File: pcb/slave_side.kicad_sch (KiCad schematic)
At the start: 2 parts, among them J6 AudioJack4

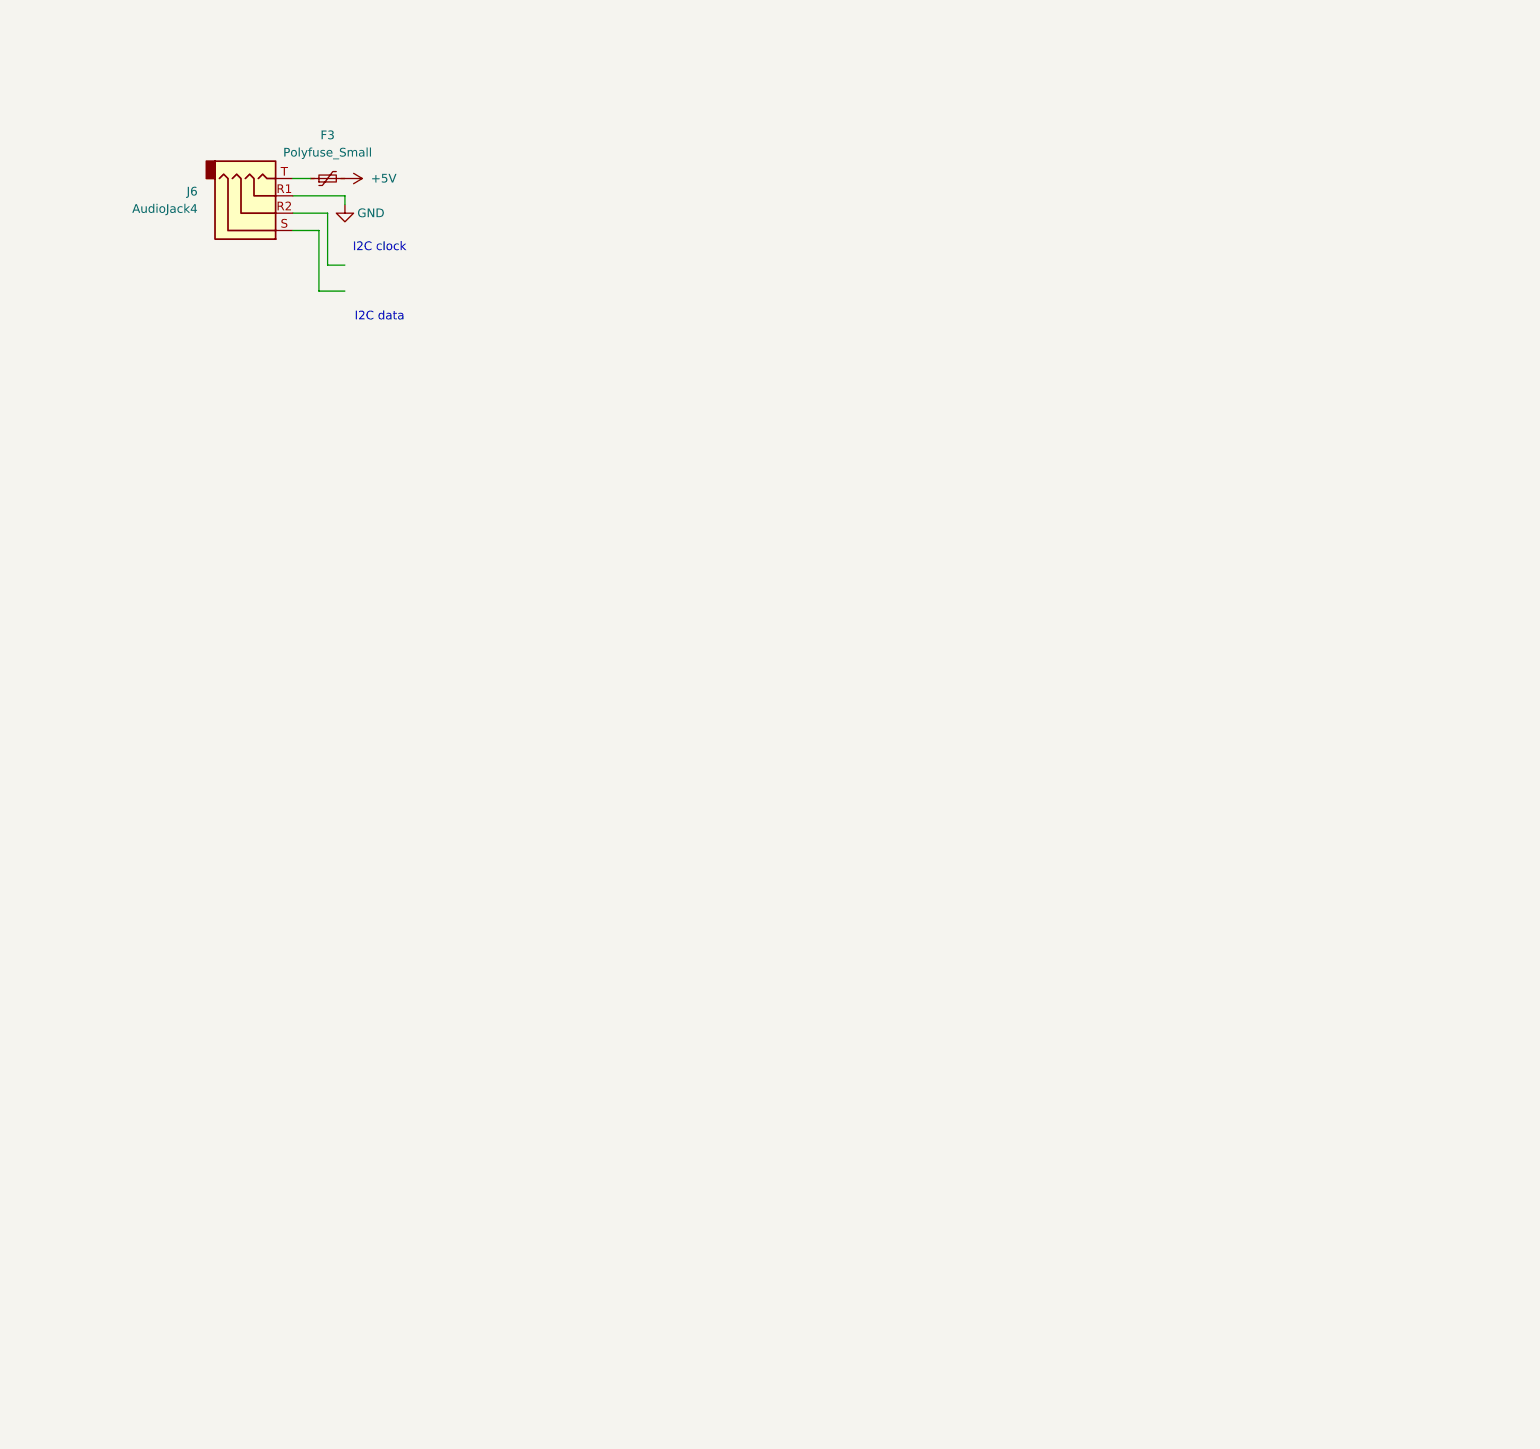
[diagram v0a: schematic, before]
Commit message: feat: Further develop right side
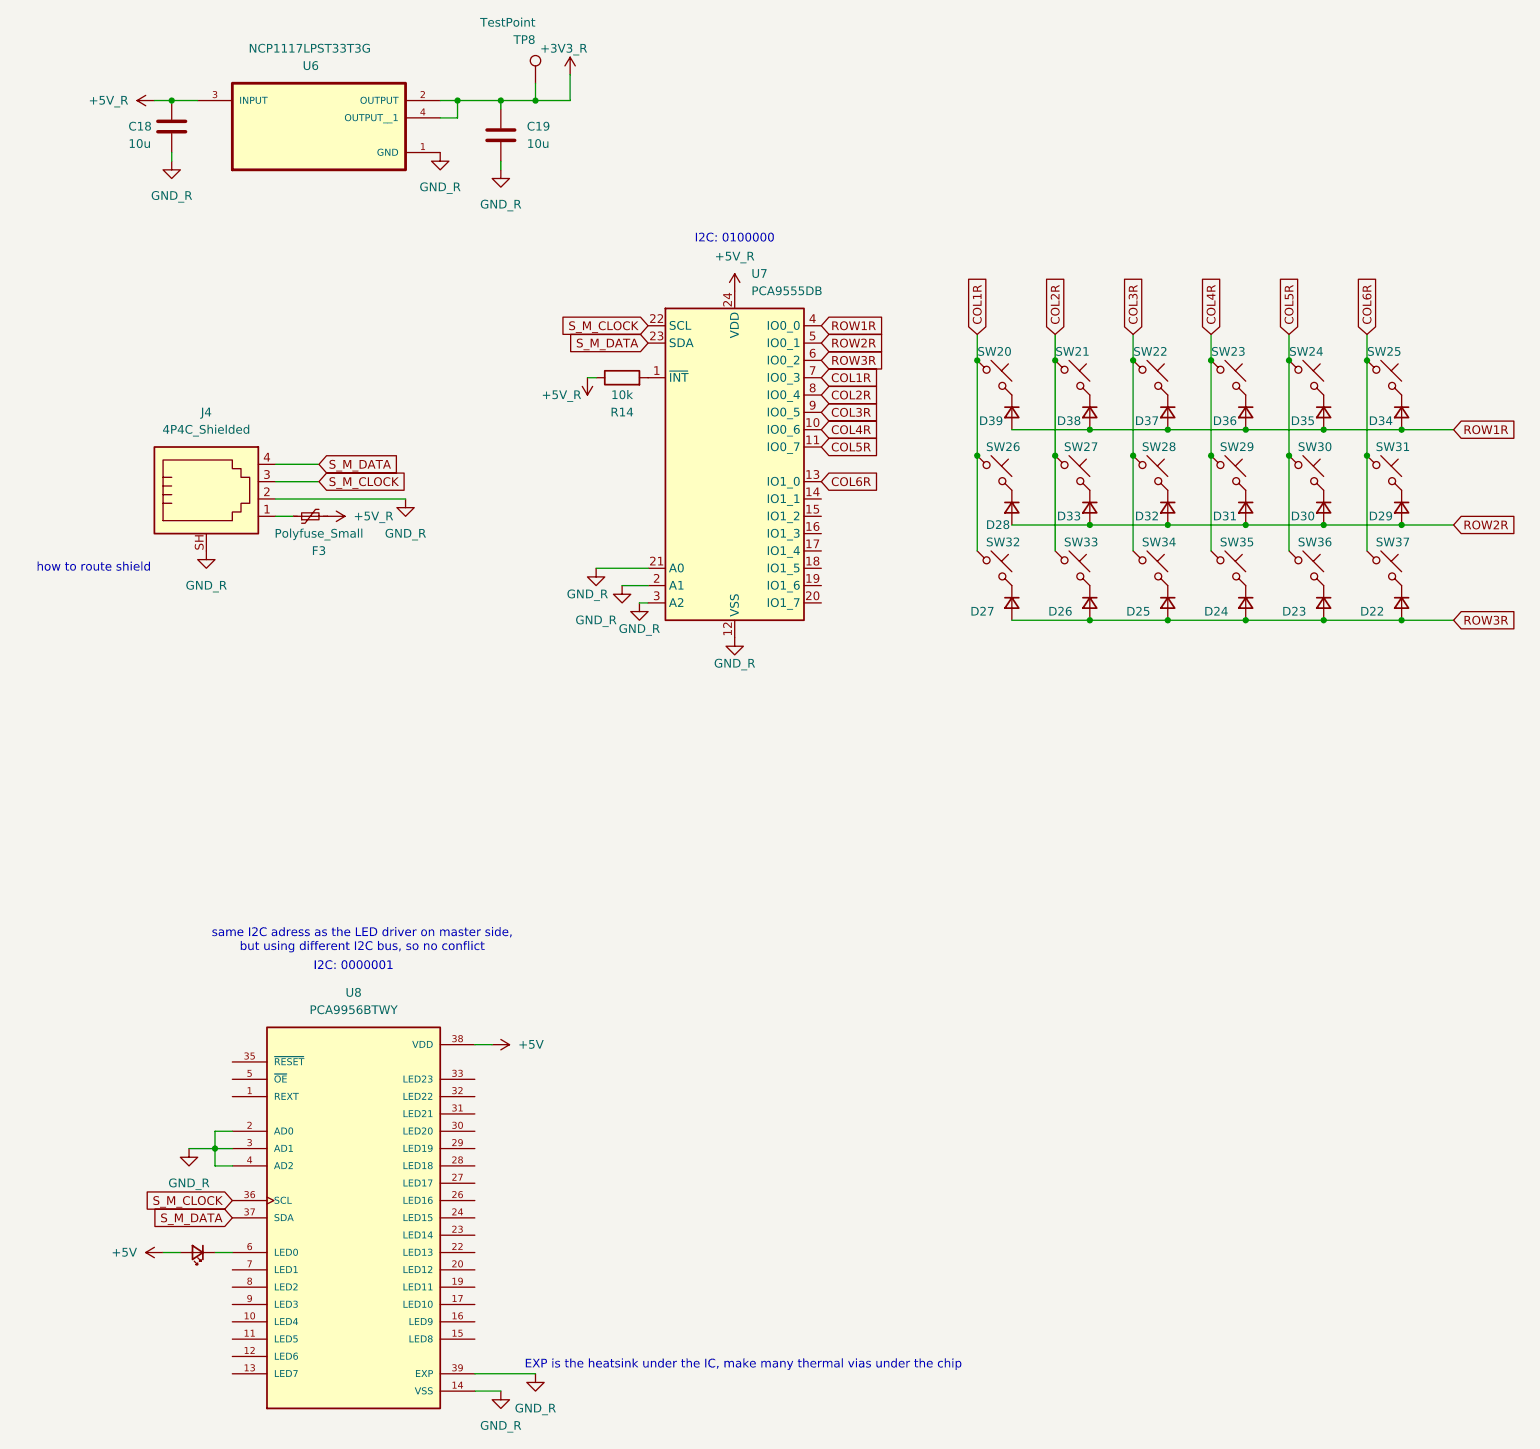
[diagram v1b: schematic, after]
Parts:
- removed J6: AudioJack4, Connector_Audio:Jack_3.5mm_CUI_SJ-3523-SMT_Horizontal, symbol Connector_Audio:AudioJack4
- added C18, C19: 10u, Capacitor_SMD:C_0805_2012Metric, symbol Device:C
- added D22, D23, D24, D25, D26, D27, D28, D29, D30, D31, D32, D33, D34, D35, D36, D37, D38, D39: D_Small, symbol Device:D_Small
- added D40: LED_Small, symbol Device:LED_Small
- added J4: 4P4C_Shielded, Connector_RJ:RJ9_Evercom_5301-440xxx_Horizontal, symbol Connector:4P4C_Shielded
- added R14: 10k, symbol library:R
- added SW20, SW21, SW22, SW23, SW24, SW25, SW26, SW27, SW28, SW29, SW30, SW31, SW32, SW33, SW34, SW35, SW36, SW37: SW_Push_45deg, ai03-MX_V2:MX-Solderable-1U, symbol Switch:SW_Push_45deg
- added TP8: TestPoint, TestPoint:TestPoint_Pad_D2.0mm, symbol Connector:TestPoint
- added U6: NCP1117LPST33T3G, NCP1117LPST33T3G:SOT230P700X175-4N, symbol NCP1117LPST33T3G:NCP1117LPST33T3G
- added U7: PCA9555DB, PCA9555DB_118:SOP65P775X200-24N, symbol Interface_Expansion:PCA9555DB
- added U8: PCA9956BTWY, PCA9956BTWY:SOP50P640X110-39N, symbol PCA9956BTWY:PCA9956BTWY
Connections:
- net +5V: now also D40.2 (A), U8.38 (VDD); no longer F3.2
- net at F3.1: now also J4.1
- new net: D24.1 (K), SW35.2
- new net: D37.1 (K), SW22.2
- new net: D32.1 (K), SW28.2
- new net: D27.1 (K), SW32.2
- new net: D34.1 (K), SW25.2
- new net: D40.1 (K), U8.6 (LED0)
- new net: D26.1 (K), SW33.2
- new net: D39.1 (K), SW20.2
- new net: D38.1 (K), SW21.2
- new net: D23.1 (K), SW36.2
- new net: D30.1 (K), SW30.2
- new net: D36.1 (K), SW23.2
- new net: D25.1 (K), SW34.2
- new net: D33.1 (K), SW27.2
- new net: D31.1 (K), SW29.2
- new net: R14.2, U7.1 (~{INT})
- new net: D28.1 (K), SW26.2
- new net: D35.1 (K), SW24.2
- new net: D22.1 (K), SW37.2
- new net: D29.1 (K), SW31.2
- new net +3V3_R: C19.1, TP8.1, U6.2 (OUTPUT), U6.4 (OUTPUT__1)
- new net +5V_R: C18.1, F3.2, R14.1, U6.3 (INPUT), U7.24 (VDD)
- new net COL1R: SW20.1, SW26.1, SW32.1, U7.7 (IO0_3)
- new net COL2R: SW21.1, SW27.1, SW33.1, U7.8 (IO0_4)
- new net COL3R: SW22.1, SW28.1, SW34.1, U7.9 (IO0_5)
- new net COL4R: SW23.1, SW29.1, SW35.1, U7.10 (IO0_6)
- new net COL5R: SW24.1, SW30.1, SW36.1, U7.11 (IO0_7)
- new net COL6R: SW25.1, SW31.1, SW37.1, U7.13 (IO1_0)
- new net GND_R: C18.2, C19.2, J4.2, J4.SH, U6.1 (GND), U7.12 (VSS), U7.2 (A1), U7.21 (A0), U7.3 (A2), U8.14 (VSS), U8.18 (VSS), U8.2 (AD0), U8.21 (VSS), U8.25 (VSS), U8.3 (AD1), U8.34 (VSS), U8.39 (EXP), U8.4 (AD2)
- new net ROW1R: D34.2 (A), D35.2 (A), D36.2 (A), D37.2 (A), D38.2 (A), D39.2 (A), U7.4 (IO0_0)
- new net ROW2R: D28.2 (A), D29.2 (A), D30.2 (A), D31.2 (A), D32.2 (A), D33.2 (A), U7.5 (IO0_1)
- new net ROW3R: D22.2 (A), D23.2 (A), D24.2 (A), D25.2 (A), D26.2 (A), D27.2 (A), U7.6 (IO0_2)
- new net S_M_CLOCK: J4.3, U7.22 (SCL), U8.36 (SCL)
- new net S_M_DATA: J4.4, U7.23 (SDA), U8.37 (SDA)
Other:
- note added: "EXP is the heatsink under the IC, make many thermal vias under the chip"
- note added: "I2C: 0000001"
- note added: "I2C: 0100000"
- note added: "how to route shield"
- note added: "same I2C adress as the LED driver on master side, but using different I2C bus, so no conflict"
- note removed: "I2C clock"
- note removed: "I2C data"
